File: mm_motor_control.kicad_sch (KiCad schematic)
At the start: 0 parts

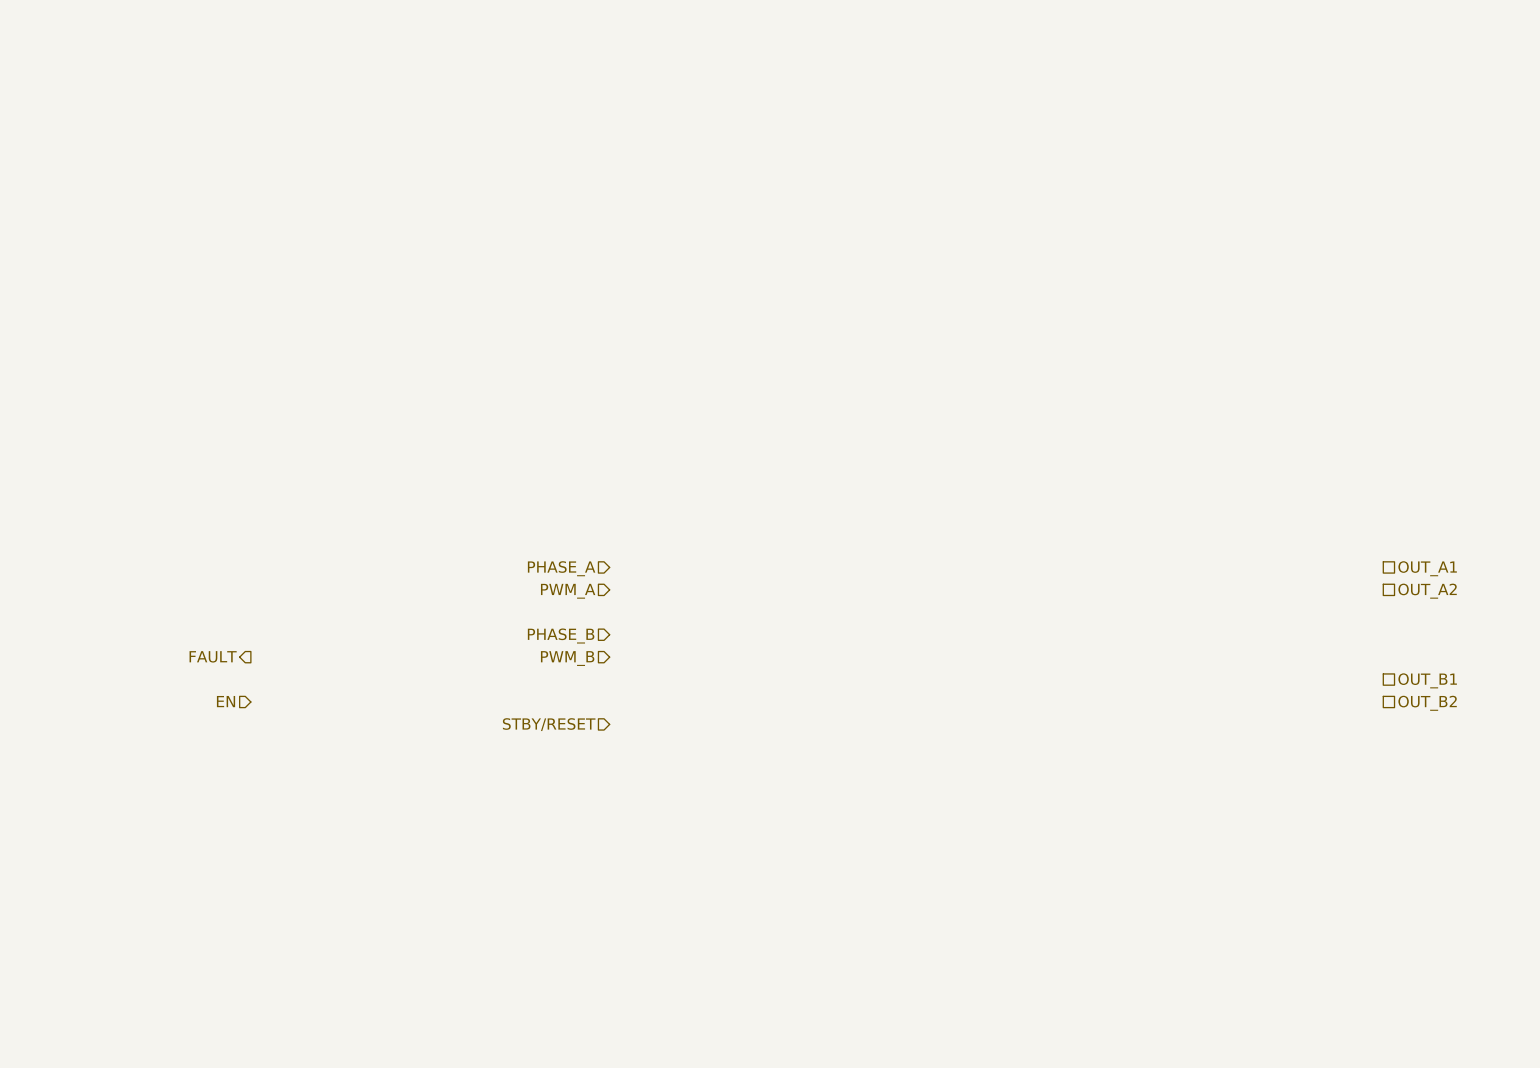
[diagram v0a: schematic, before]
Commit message: tp2
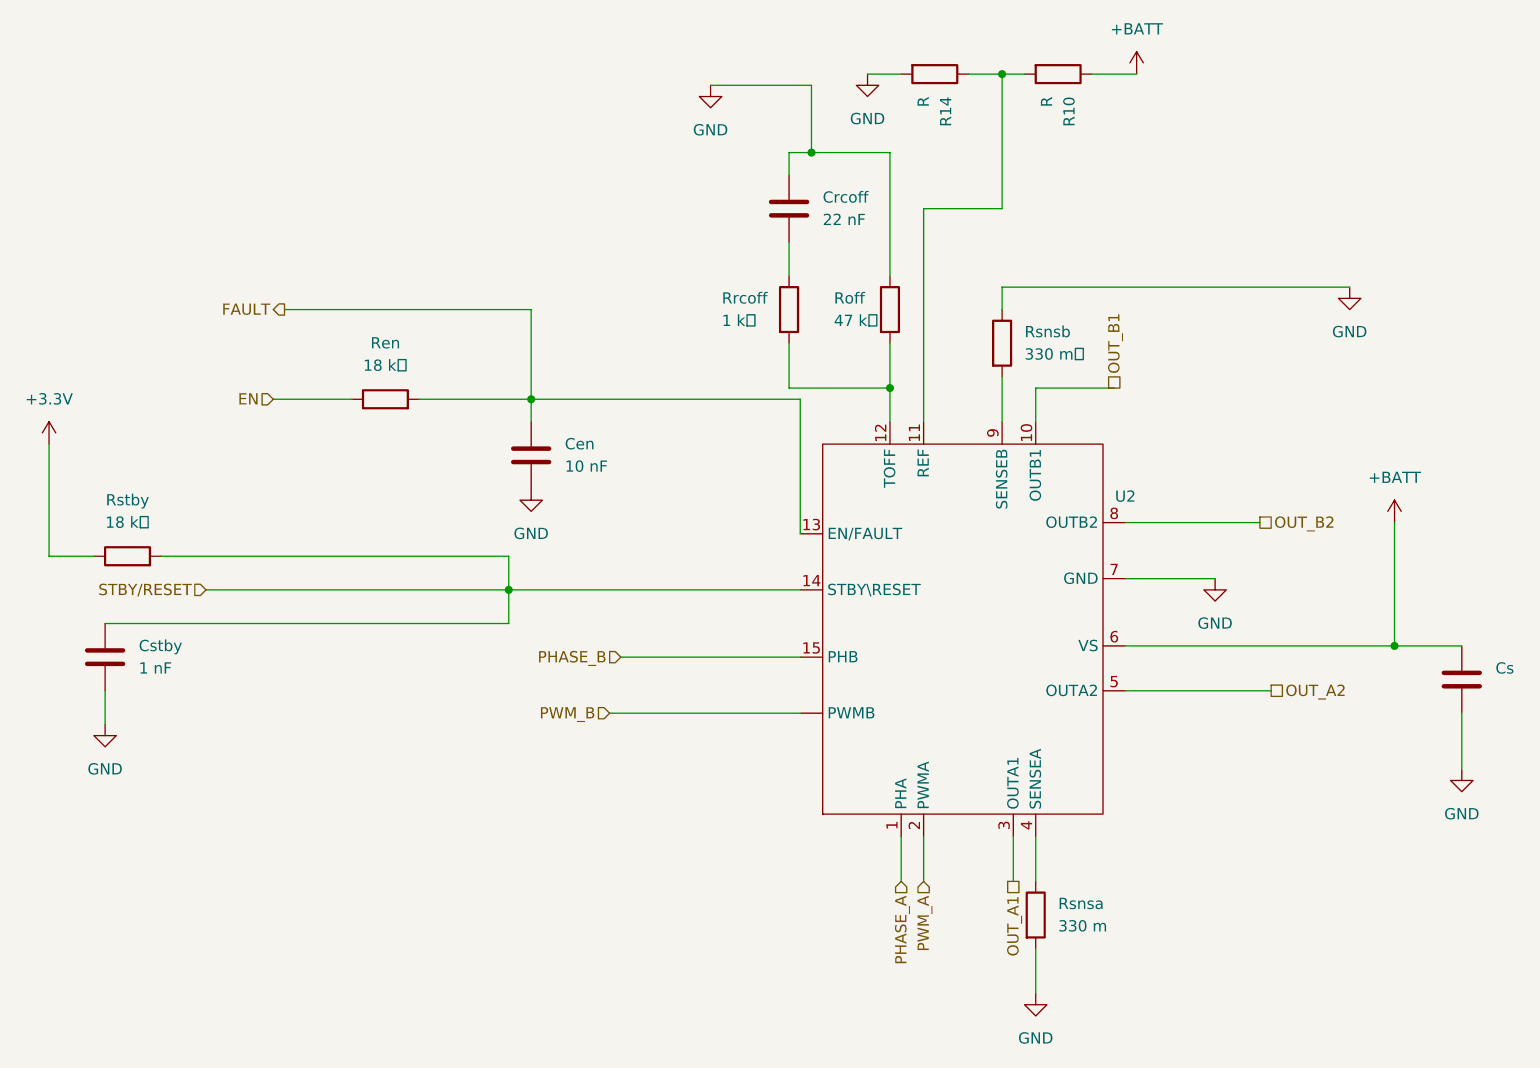
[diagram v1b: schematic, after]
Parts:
- added Cen: 10 nF, symbol Device:C
- added Crcoff: 22 nF, symbol Device:C
- added Cs: 2.2 uF, symbol Device:C
- added Cstby: 1 nF, symbol Device:C
- added R10, R14: R, symbol Device:R
- added Ren, Rstby: 18 k, symbol Device:R
- added Roff: 47 k, symbol Device:R
- added Rrcoff: 1 k, symbol Device:R
- added Rsnsa: 330 m, symbol Device:R
- added Rsnsb: 330 m, symbol Device:R
- added U2: ~, symbol STM:STSPIN240
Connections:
- net EN: now also Ren.1
- net FAULT: now also Cen.1, Ren.2, U2.13 (EN/FAULT)
- net OUT_A1: now also U2.3 (OUTA1)
- net OUT_A2: now also U2.5 (OUTA2)
- net OUT_B1: now also U2.10 (OUTB1)
- net OUT_B2: now also U2.8 (OUTB2)
- net PHASE_A: now also U2.1 (PHA)
- net PHASE_B: now also U2.15 (PHB)
- net PWM_A: now also U2.2 (PWMA)
- net PWM_B: now also U2. (PWMB)
- net STBY/RESET: now also Cstby.1, Rstby.2, U2.14 (STBY\RESET)
- new net: R10.2, R14.1, U2.11 (REF)
- new net: Rsnsa.1, U2.4 (SENSEA)
- new net: Crcoff.2, Rrcoff.1
- new net: Roff.2, Rrcoff.2, U2.12 (TOFF)
- new net: Rsnsb.2, U2.9 (SENSEB)
- new net +3.3V: Rstby.1
- new net +BATT: Cs.1, R10.1, U2.6 (VS)
- new net GND: Cen.2, Crcoff.1, Cs.2, Cstby.2, R14.2, Roff.1, Rsnsa.2, Rsnsb.1, U2.7 (GND)
